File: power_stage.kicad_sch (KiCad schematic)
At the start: 27 parts, among them J1 Input, J1 Output, Q1 IMW120R014M1H, Q2 IMW120R014M1H, Q6 2N7002BK,215, U4 TC4432VOA

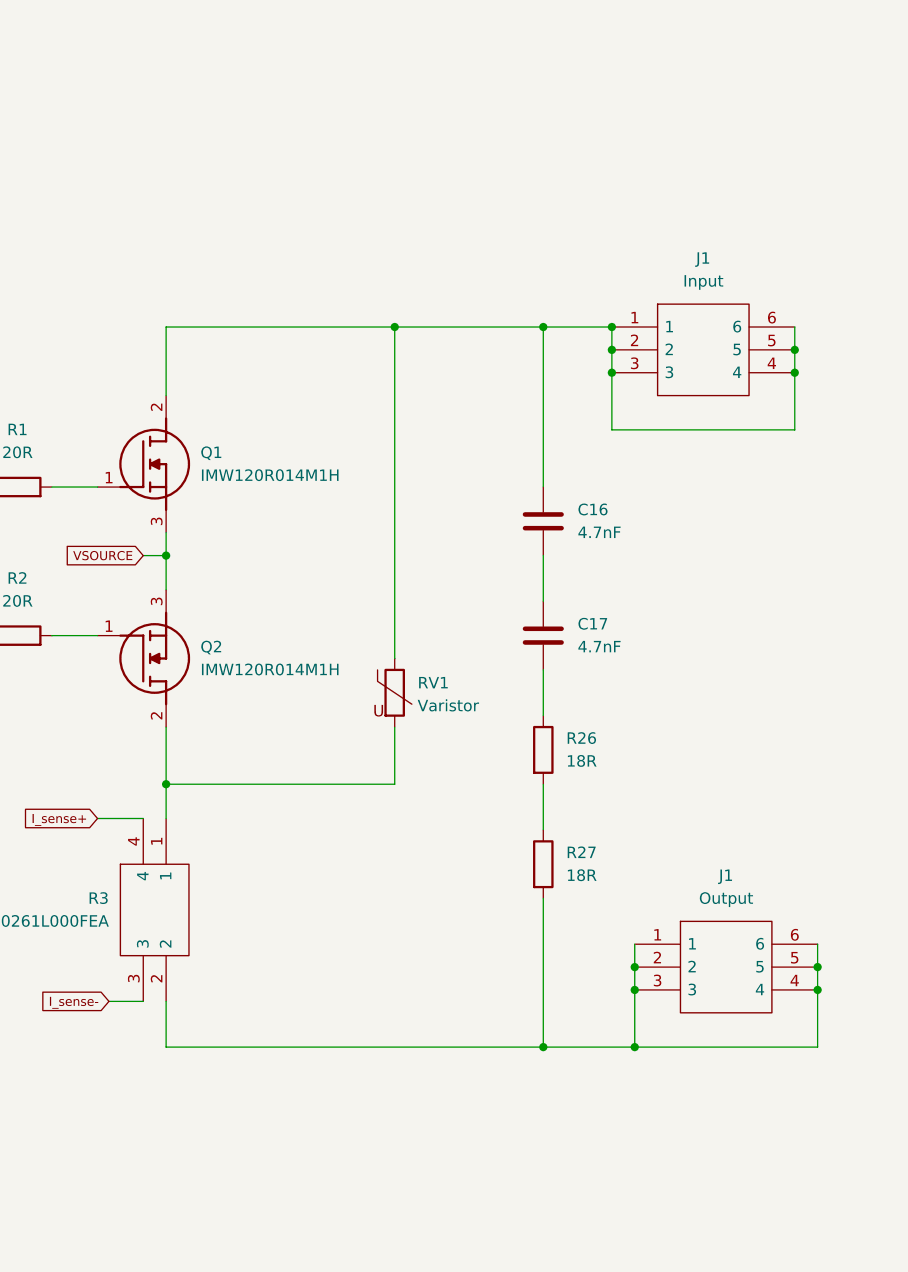
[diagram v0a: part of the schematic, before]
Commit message: design update
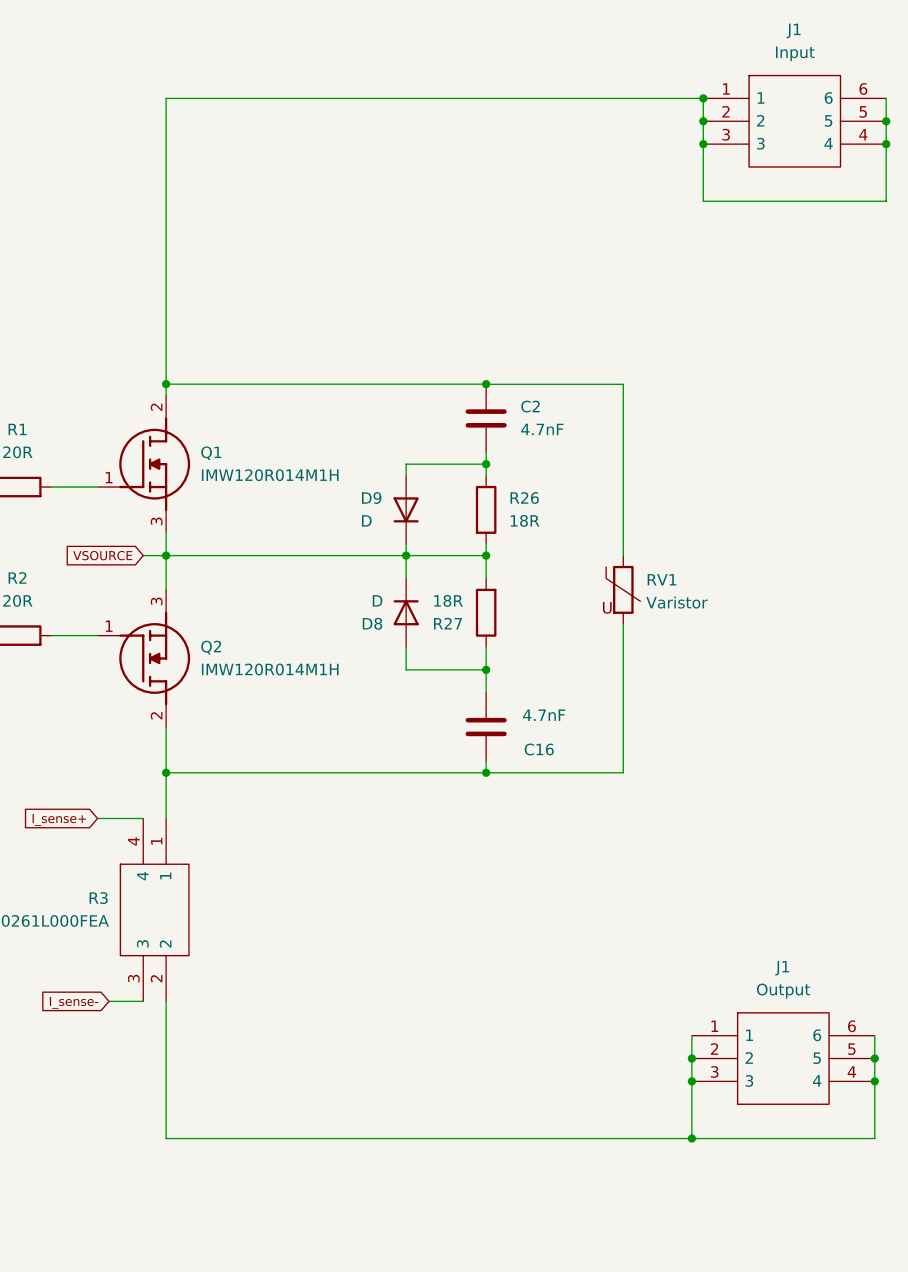
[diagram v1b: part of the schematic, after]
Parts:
- removed C17: 4.7nF, Capacitor_SMD:C_1812_4532Metric, symbol Device:C
- added C2: 4.7nF, Capacitor_SMD:C_1812_4532Metric, symbol Device:C
- added D8, D9: D, Diode_THT:D_DO-201AE_P12.70mm_Horizontal, symbol Device:D
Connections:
- net VSOURCE: now also R26.2, R27.2, D8.1 (K), D9.1 (K)
- net at R26.1: now also C2.2, D9.2 (A)
- net at R27.1: now also C16.2, D8.2 (A); no longer R26.2
- net at J1.1, J1.2, J1.3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: no longer R27.2
- net at Q2.2 (D), R3.1, RV1.2: now also C16.1
- net at J1.1, J1.2, J1.3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: now also C2.1; no longer C16.1
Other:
- moved on the sheet: J1, RV1
